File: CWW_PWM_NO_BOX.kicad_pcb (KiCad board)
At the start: 2 copper layers, 28 x 28 mm, 18 parts, among them J1 RJ12, P1 CONN_01X04, P2 CONN_01X02, U1 BP1360, U2 BP1360

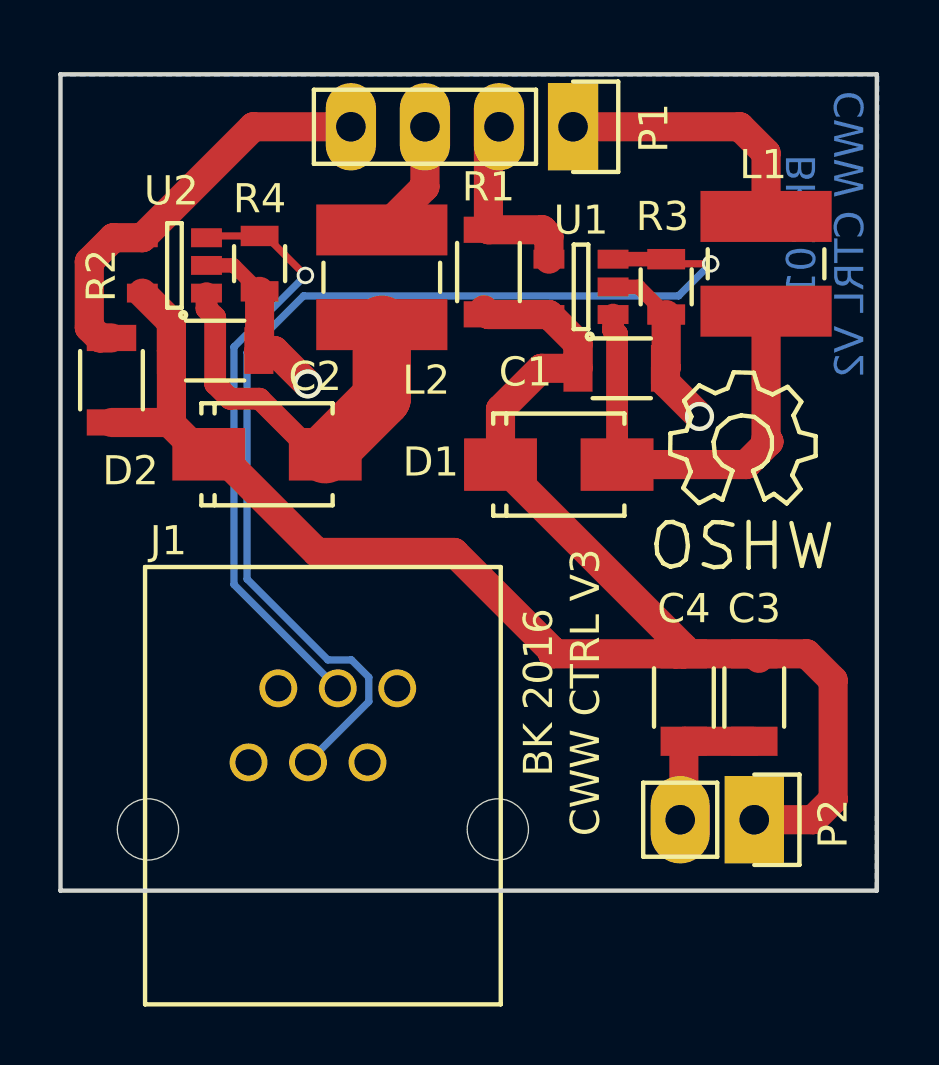
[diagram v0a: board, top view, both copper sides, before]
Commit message: pcb change
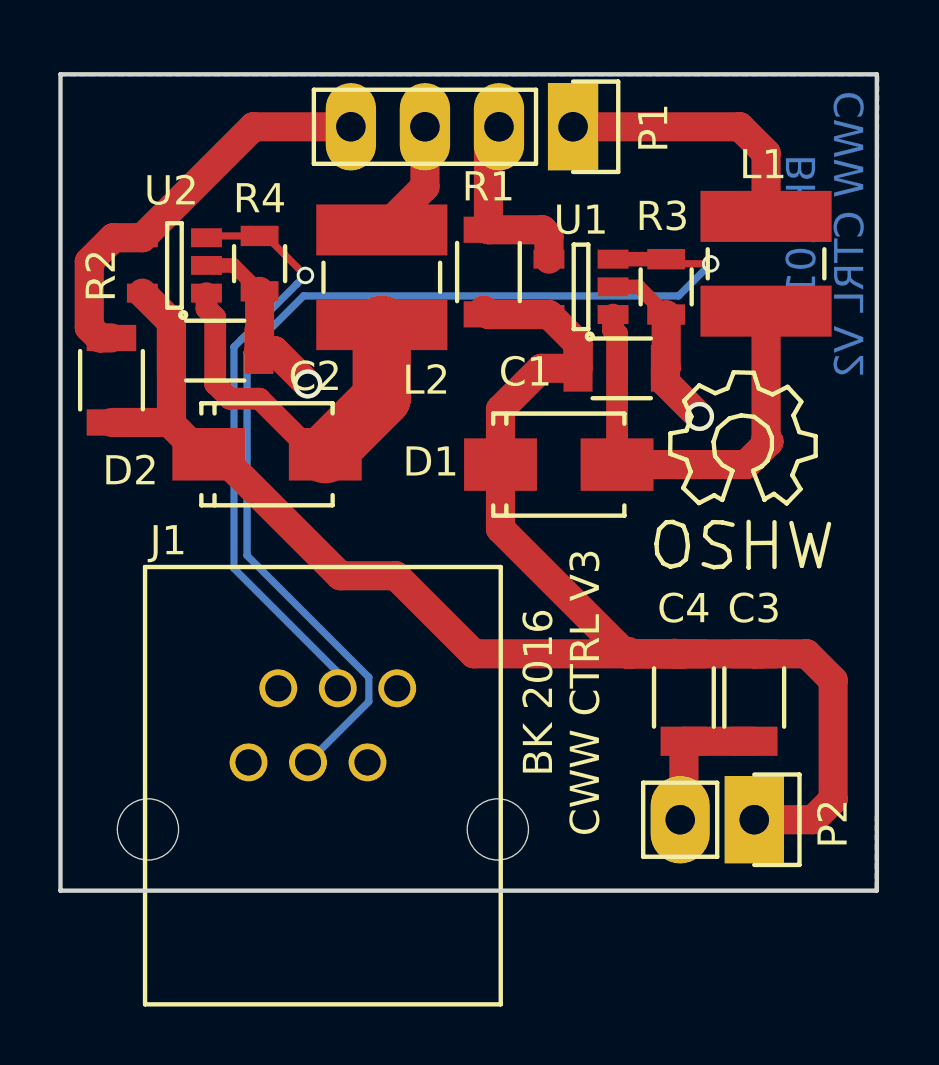
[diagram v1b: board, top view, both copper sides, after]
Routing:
- net /VIN: track 60.4 -> 61.4 mm
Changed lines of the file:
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@@
 (kicad_pcb (version 4) (host pcbnew 4.0.2-stable)
   (general
-    (links 0)
-    (no_connects 5)
-    (area 139.924999 61.924999 168.075001 90.075001)
+    (links 34)
+    (no_connects 0)
+    (area 137.5 58.691666 175.818215 94.175001)
     (thickness 1.6)
     (drawings 8)
-    (tracks 106)
+    (tracks 109)
     (zones 0)
     (modules 18)
@@
   (segment (start 145.008 68.556) (end 145.94 68.556) (width 0.5) (layer F.Cu) (net 1))
   (segment (start 145.94 68.556) (end 146.829 69.445) (width 0.5) (layer F.Cu) (net 1))
-  (segment (start 161.382 81.877) (end 161.382 81.67698) (width 1) (layer F.Cu) (net 2))
-  (segment (start 161.382 81.67698) (end 155.09202 75.387) (width 1) (layer F.Cu) (net 2))
-  (segment (start 153.5 78.4) (end 148.80027 78.4) (width 1) (layer F.Cu) (net 2))
-  (segment (start 148.80027 78.4) (end 145.43327 75.033) (width 1) (layer F.Cu) (net 2))
+  (segment (start 161.382 81.877) (end 154.177 81.877) (width 1) (layer F.Cu) (net 2))
+  (segment (start 154.177 81.877) (end 151.5 79.2) (width 1) (layer F.Cu) (net 2))
+  (segment (start 151.5 79.2) (end 149.60027 79.2) (width 1) (layer F.Cu) (net 2))
+  (segment (start 149.60027 79.2) (end 145.43327 75.033) (width 1) (layer F.Cu) (net 2))
   (segment (start 145.43327 75.033) (end 145.08402 75.033) (width 1) (layer F.Cu) (net 2))
-  (segment (start 156.877 81.777) (end 153.5 78.4) (width 1) (layer F.Cu) (net 2))
-  (segment (start 156.877 81.877) (end 156.877 81.777) (width 1) (layer F.Cu) (net 2))
-  (segment (start 161.382 81.877) (end 156.877 81.877) (width 1) (layer F.Cu) (net 2))
+  (segment (start 159.582 81.877) (end 159.377 81.877) (width 1) (layer F.Cu) (net 2))
+  (segment (start 159.377 81.877) (end 155.09202 77.59202) (width 1) (layer F.Cu) (net 2))
+  (segment (start 155.09202 77.59202) (end 155.09202 77.28743) (width 1) (layer F.Cu) (net 2))
+  (segment (start 155.09202 77.28743) (end 155.09202 75.387) (width 1) (layer F.Cu) (net 2))
+  (segment (start 159.582 81.877) (end 159.505 81.8) (width 1) (layer F.Cu) (net 2))
+  (segment (start 161.382 81.877) (end 159.582 81.877) (width 1) (layer F.Cu) (net 2))
   (segment (start 166.5 82.782) (end 166.5 86.879) (width 1) (layer F.Cu) (net 2))
   (segment (start 166.5 86.879) (end 165.811 87.568) (width 1) (layer F.Cu) (net 2))
@@
   (segment (start 163.795 81.877) (end 165.595 81.877) (width 1) (layer F.Cu) (net 2))
   (segment (start 165.595 81.877) (end 166.5 82.782) (width 1) (layer F.Cu) (net 2))
-  (segment (start 163.951 82.033) (end 163.795 81.877) (width 1) (layer F.Cu) (net 2))
   (segment (start 161.382 81.877) (end 161.082 81.877) (width 1) (layer F.Cu) (net 2))
   (segment (start 161.082 81.877) (end 161.058 81.853) (width 1) (layer F.Cu) (net 2))
@@
   (segment (start 140.987 68.429) (end 141.81 67.606) (width 1) (layer F.Cu) (net 8))
   (segment (start 141.81 67.606) (end 142.808 67.606) (width 1) (layer F.Cu) (net 8))
+  (segment (start 149.51 83.06) (end 149.51 82.51) (width 0.25) (layer B.Cu) (net 9))
+  (segment (start 149.51 82.51) (end 145.949989 78.949989) (width 0.25) (layer B.Cu) (net 9))
+  (segment (start 145.949989 78.949989) (end 145.949989 71.35001) (width 0.25) (layer B.Cu) (net 9))
+  (segment (start 145.949989 71.35001) (end 146.213601 71.086399) (width 0.25) (layer B.Cu) (net 9))
+  (segment (start 146.213601 71.086399) (end 148.100001 69.199999) (width 0.25) (layer B.Cu) (net 9))
+  (segment (start 148.100001 69.199999) (end 148.4 68.9) (width 0.25) (layer B.Cu) (net 9))
   (segment (start 146.9 67.4) (end 146.9 67.474) (width 0.25) (layer F.Cu) (net 9))
   (segment (start 146.9 67.474) (end 146.829 67.545) (width 0.25) (layer F.Cu) (net 9))
   (segment (start 148.4 68.9) (end 146.9 67.4) (width 0.25) (layer F.Cu) (net 9))
   (via (at 148.4 68.9) (size 0.6) (drill 0.4) (layers F.Cu B.Cu) (net 9))
-  (segment (start 145.95 71.35) (end 148.4 68.9) (width 0.25) (layer B.Cu) (net 9))
-  (segment (start 149.51 83.06) (end 145.95 79.5) (width 0.25) (layer B.Cu) (net 9))
-  (segment (start 145.95 79.5) (end 145.95 71.35) (width 0.25) (layer B.Cu) (net 9))
   (segment (start 147.129 67.545) (end 146.829 67.545) (width 0.25) (layer F.Cu) (net 9))
   (segment (start 146.829 67.545) (end 145.069 67.545) (width 0.25) (layer F.Cu) (net 9))
@@
   (segment (start 148.49 85.6) (end 150.574999 83.515001) (width 0.25) (layer B.Cu) (net 10))
   (segment (start 150.574999 83.515001) (end 150.574999 82.681997) (width 0.25) (layer B.Cu) (net 10))
-  (segment (start 150.574999 82.681997) (end 149.978001 82.084999) (width 0.25) (layer B.Cu) (net 10))
-  (segment (start 149.978001 82.084999) (end 149.171409 82.084999) (width 0.25) (layer B.Cu) (net 10))
-  (segment (start 149.171409 82.084999) (end 146.4 79.31359) (width 0.25) (layer B.Cu) (net 10))
-  (segment (start 146.4 79.31359) (end 146.4 71.53641) (width 0.25) (layer B.Cu) (net 10))
+  (segment (start 150.574999 82.681997) (end 146.4 78.506998) (width 0.25) (layer B.Cu) (net 10))
+  (segment (start 146.4 78.506998) (end 146.4 71.53641) (width 0.25) (layer B.Cu) (net 10))
   (segment (start 146.4 71.53641) (end 148.33641 69.6) (width 0.25) (layer B.Cu) (net 10))
   (segment (start 148.33641 69.6) (end 161.2 69.6) (width 0.25) (layer B.Cu) (net 10))
